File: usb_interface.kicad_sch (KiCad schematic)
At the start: 57 parts, among them J7 USB4105-GF-A-060, J8 PD_I2C DEBUG, Q1 CSD23280F3, Q2 CSD15380F3, Q3 CSD23280F3, Q4 CSD15380F3, U21 M24512-DFMC6TG, U3 TVS2200DRV, U4 TPD8S300A, U5 TPS25751DREFR

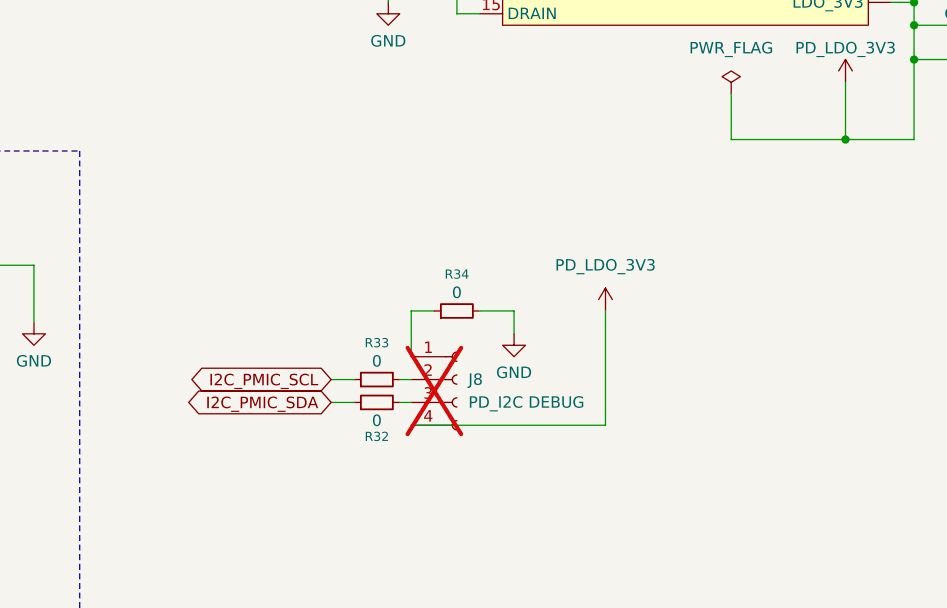
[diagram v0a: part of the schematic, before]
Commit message: replot schematic
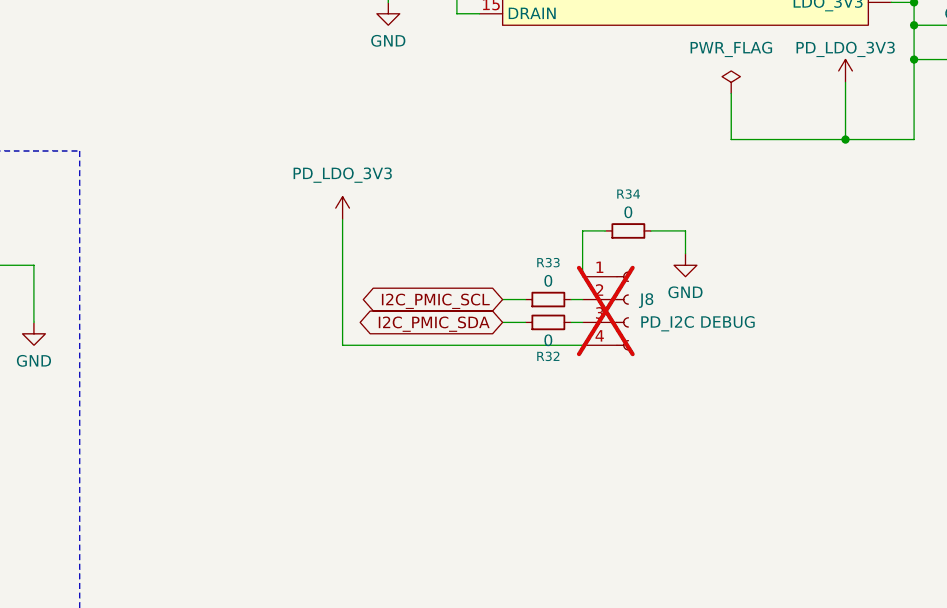
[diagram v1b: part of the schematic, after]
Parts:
- J8: now in the parts list
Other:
- moved on the sheet: J8, R32, R33, R34
